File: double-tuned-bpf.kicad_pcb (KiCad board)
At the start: 2 copper layers, 52.4 x 15.6 mm, 12 parts, among them J1 PCB_SMA_EDGE, J2 PCB_SMA_EDGE, J3 Conn_01x03_Female, J4 Conn_01x03_Female, T1 6:31, T2 31:6

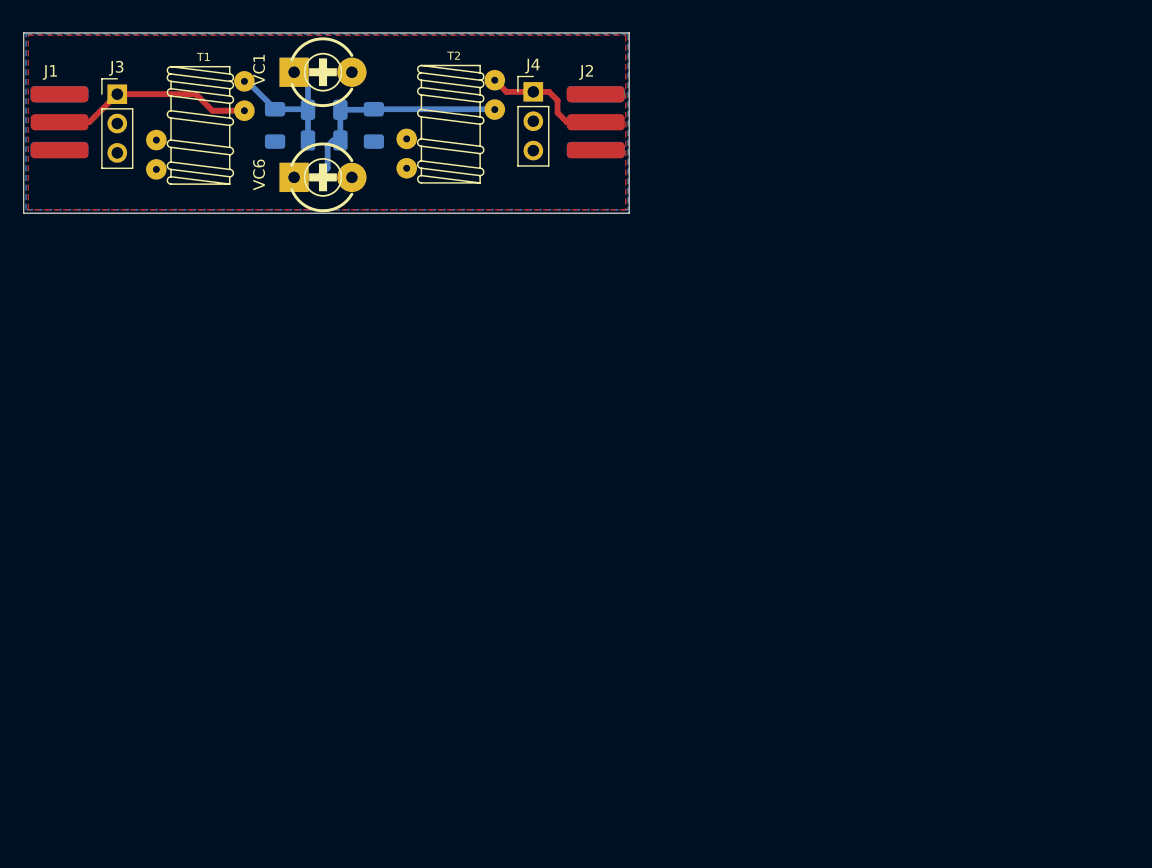
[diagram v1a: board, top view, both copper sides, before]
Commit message: gg
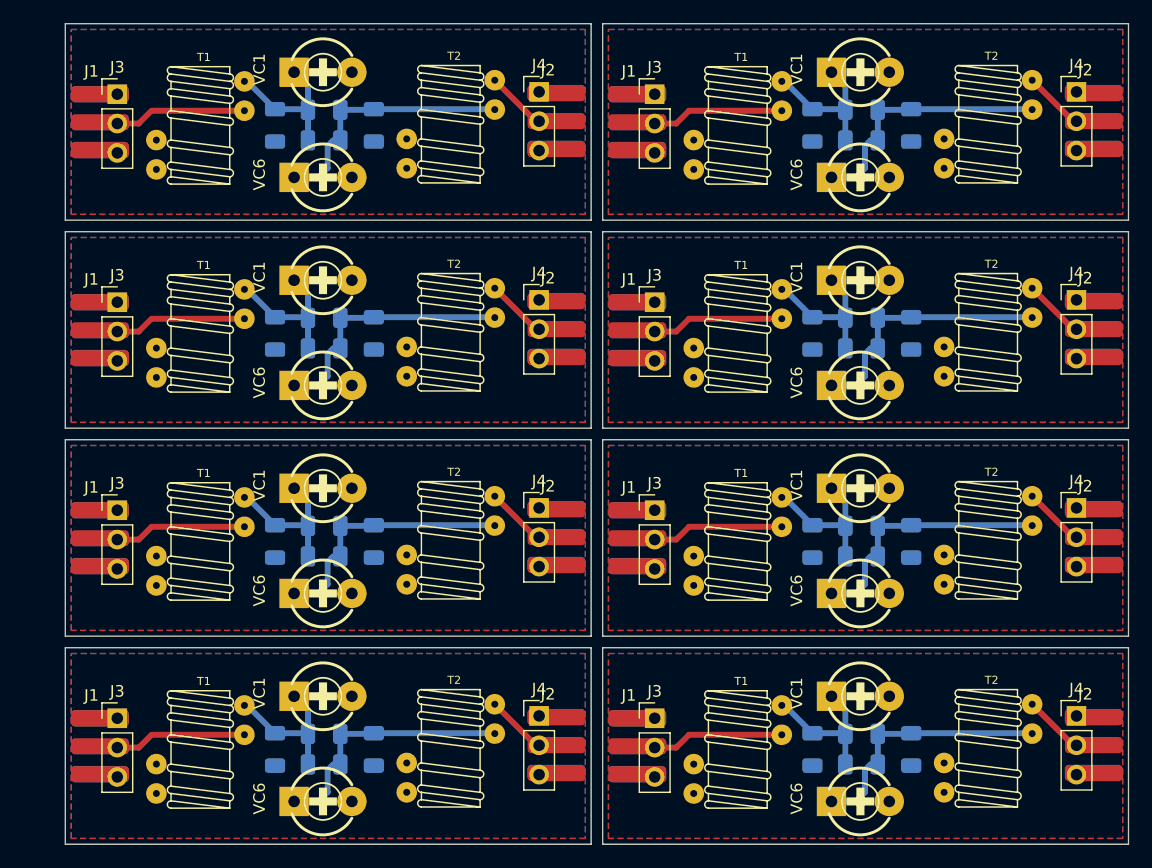
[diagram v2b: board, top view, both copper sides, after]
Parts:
- added C2: 150pF, Xenir:Capacitor 1206, B.Cu at (124.9, 133.8)
- added C2: 150pF, Xenir:Capacitor 1206, B.Cu at (171.4, 133.8)
- added C2: 150pF, Xenir:Capacitor 1206, B.Cu at (124.9, 151.8)
- added C2: 150pF, Xenir:Capacitor 1206, B.Cu at (171.4, 151.8)
- added C2: 150pF, Xenir:Capacitor 1206, B.Cu at (124.9, 115.8)
- added C2: 150pF, Xenir:Capacitor 1206, B.Cu at (171.4, 115.8)
- added C2: 150pF, Xenir:Capacitor 1206, B.Cu at (171.4, 97.8)
- added C3: 5pF, Xenir:Capacitor 1206, B.Cu at (173.4, 137.3)
- added C3: 5pF, Xenir:Capacitor 1206, B.Cu at (126.9, 137.3)
- added C3: 5pF, Xenir:Capacitor 1206, B.Cu at (173.4, 155.3)
- added C3: 5pF, Xenir:Capacitor 1206, B.Cu at (126.9, 155.3)
- added C3: 5pF, Xenir:Capacitor 1206, B.Cu at (173.4, 119.3)
- added C3: 5pF, Xenir:Capacitor 1206, B.Cu at (126.9, 119.3)
- added C3: 5pF, Xenir:Capacitor 1206, B.Cu at (173.4, 101.3)
- added C4: 10pF, Xenir:Capacitor 1206, B.Cu at (173.4, 134.7)
- added C4: 10pF, Xenir:Capacitor 1206, B.Cu at (126.9, 134.7)
- added C4: 10pF, Xenir:Capacitor 1206, B.Cu at (126.9, 152.7)
- added C4: 10pF, Xenir:Capacitor 1206, B.Cu at (173.4, 152.7)
- added C4: 10pF, Xenir:Capacitor 1206, B.Cu at (173.4, 116.7)
- added C4: 10pF, Xenir:Capacitor 1206, B.Cu at (126.9, 116.7)
- added C4: 10pF, Xenir:Capacitor 1206, B.Cu at (173.4, 98.7)
- added C5: 150pF, Xenir:Capacitor 1206, B.Cu at (133.4, 133.8)
- added C5: 150pF, Xenir:Capacitor 1206, B.Cu at (179.9, 133.8)
- added C5: 150pF, Xenir:Capacitor 1206, B.Cu at (133.4, 151.8)
- added C5: 150pF, Xenir:Capacitor 1206, B.Cu at (179.9, 151.8)
- added C5: 150pF, Xenir:Capacitor 1206, B.Cu at (133.4, 115.8)
- added C5: 150pF, Xenir:Capacitor 1206, B.Cu at (179.9, 115.8)
- added C5: 150pF, Xenir:Capacitor 1206, B.Cu at (179.9, 97.8)
- added J1: PCB_SMA_EDGE, Xenir:PCB-SMA-EDGE, F.Cu at (154.0, 146.4)
- added J1: PCB_SMA_EDGE, Xenir:PCB-SMA-EDGE, F.Cu at (107.5, 128.4)
- added J1: PCB_SMA_EDGE, Xenir:PCB-SMA-EDGE, F.Cu at (107.5, 146.4)
- added J1: PCB_SMA_EDGE, Xenir:PCB-SMA-EDGE, F.Cu at (154.0, 128.4)
- added J1: PCB_SMA_EDGE, Xenir:PCB-SMA-EDGE, F.Cu at (107.5, 110.4)
- added J1: PCB_SMA_EDGE, Xenir:PCB-SMA-EDGE, F.Cu at (154.0, 110.4)
- added J1: PCB_SMA_EDGE, Xenir:PCB-SMA-EDGE, F.Cu at (154.0, 92.4)
- added J2: PCB_SMA_EDGE, Xenir:PCB-SMA-EDGE, F.Cu at (193.5, 128.3)
- added J2: PCB_SMA_EDGE, Xenir:PCB-SMA-EDGE, F.Cu at (147.0, 128.3)
- added J2: PCB_SMA_EDGE, Xenir:PCB-SMA-EDGE, F.Cu at (193.5, 146.3)
- added J2: PCB_SMA_EDGE, Xenir:PCB-SMA-EDGE, F.Cu at (147.0, 146.3)
- added J2: PCB_SMA_EDGE, Xenir:PCB-SMA-EDGE, F.Cu at (193.5, 110.3)
- added J2: PCB_SMA_EDGE, Xenir:PCB-SMA-EDGE, F.Cu at (147.0, 110.3)
- added J2: PCB_SMA_EDGE, Xenir:PCB-SMA-EDGE, F.Cu at (193.5, 92.3)
- added J3: Conn_01x03_Female, Connector_PinHeader_2.54mm:PinHeader_1x03_P2.54mm_Vertical, F.Cu at (109.0, 131.1)
- added J3: Conn_01x03_Female, Connector_PinHeader_2.54mm:PinHeader_1x03_P2.54mm_Vertical, F.Cu at (155.5, 149.1)
- added J3: Conn_01x03_Female, Connector_PinHeader_2.54mm:PinHeader_1x03_P2.54mm_Vertical, F.Cu at (109.0, 149.1)
- added J3: Conn_01x03_Female, Connector_PinHeader_2.54mm:PinHeader_1x03_P2.54mm_Vertical, F.Cu at (155.5, 131.1)
- added J3: Conn_01x03_Female, Connector_PinHeader_2.54mm:PinHeader_1x03_P2.54mm_Vertical, F.Cu at (109.0, 113.1)
- added J3: Conn_01x03_Female, Connector_PinHeader_2.54mm:PinHeader_1x03_P2.54mm_Vertical, F.Cu at (155.5, 113.1)
- added J3: Conn_01x03_Female, Connector_PinHeader_2.54mm:PinHeader_1x03_P2.54mm_Vertical, F.Cu at (155.5, 95.1)
- added J4: Conn_01x03_Female, Connector_PinHeader_2.54mm:PinHeader_1x03_P2.54mm_Vertical, F.Cu at (192.0, 130.9)
- added J4: Conn_01x03_Female, Connector_PinHeader_2.54mm:PinHeader_1x03_P2.54mm_Vertical, F.Cu at (145.5, 130.9)
- added J4: Conn_01x03_Female, Connector_PinHeader_2.54mm:PinHeader_1x03_P2.54mm_Vertical, F.Cu at (192.0, 148.9)
- added J4: Conn_01x03_Female, Connector_PinHeader_2.54mm:PinHeader_1x03_P2.54mm_Vertical, F.Cu at (145.5, 148.9)
- added J4: Conn_01x03_Female, Connector_PinHeader_2.54mm:PinHeader_1x03_P2.54mm_Vertical, F.Cu at (192.0, 112.9)
- added J4: Conn_01x03_Female, Connector_PinHeader_2.54mm:PinHeader_1x03_P2.54mm_Vertical, F.Cu at (145.5, 112.9)
- added J4: Conn_01x03_Female, Connector_PinHeader_2.54mm:PinHeader_1x03_P2.54mm_Vertical, F.Cu at (192.0, 94.9)
- added T1: 6:31, Xenir:T37 Transformer, F.Cu at (116.2, 126.8)
- added T1: 6:31, Xenir:T37 Transformer, F.Cu at (162.7, 126.8)
- added T1: 6:31, Xenir:T37 Transformer, F.Cu at (116.2, 144.8)
- added T1: 6:31, Xenir:T37 Transformer, F.Cu at (162.7, 144.8)
- added T1: 6:31, Xenir:T37 Transformer, F.Cu at (116.2, 108.8)
- added T1: 6:31, Xenir:T37 Transformer, F.Cu at (162.7, 108.8)
- added T1: 6:31, Xenir:T37 Transformer, F.Cu at (162.7, 90.8)
- added T2: 31:6, Xenir:T37 Transformer, F.Cu at (137.9, 126.7)
- added T2: 31:6, Xenir:T37 Transformer, F.Cu at (137.9, 144.7)
- added T2: 31:6, Xenir:T37 Transformer, F.Cu at (184.4, 144.7)
- added T2: 31:6, Xenir:T37 Transformer, F.Cu at (184.4, 126.7)
- added T2: 31:6, Xenir:T37 Transformer, F.Cu at (137.9, 108.7)
- added T2: 31:6, Xenir:T37 Transformer, F.Cu at (184.4, 108.7)
- added T2: 31:6, Xenir:T37 Transformer, F.Cu at (184.4, 90.7)
- added VC1: 40pF, Xenir:trimcap, F.Cu at (120.3, 129.2)
- added VC1: 40pF, Xenir:trimcap, F.Cu at (166.8, 147.2)
- added VC1: 40pF, Xenir:trimcap, F.Cu at (120.3, 147.2)
- added VC1: 40pF, Xenir:trimcap, F.Cu at (166.8, 129.2)
- added VC1: 40pF, Xenir:trimcap, F.Cu at (120.3, 111.2)
- added VC1: 40pF, Xenir:trimcap, F.Cu at (166.8, 111.2)
- added VC1: 40pF, Xenir:trimcap, F.Cu at (166.8, 93.2)
- added VC6: 40pF, Xenir:trimcap, F.Cu at (120.3, 138.3)
- added VC6: 40pF, Xenir:trimcap, F.Cu at (166.8, 138.3)
- added VC6: 40pF, Xenir:trimcap, F.Cu at (166.8, 156.3)
- added VC6: 40pF, Xenir:trimcap, F.Cu at (120.3, 156.3)
- added VC6: 40pF, Xenir:trimcap, F.Cu at (120.3, 120.3)
- added VC6: 40pF, Xenir:trimcap, F.Cu at (166.8, 120.3)
- added VC6: 40pF, Xenir:trimcap, F.Cu at (166.8, 102.3)
- moved J1 3.50 mm to (107.5, 92.4)
- moved J2 3.40 mm to (147.0, 92.3)
- moved J4 0.50 mm to (145.5, 94.9)
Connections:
- J3 pad 1: Input -> GND
- J3 pad 2: (no net) -> Input
- J4 pad 1: Output -> GND
- J4 pad 2: (no net) -> Output
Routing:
- net (no net): track 0.00 -> 366.6 mm
- net Input: track 17.6 -> 11.5 mm
- net Output: track 10.9 -> 5.31 mm
- added copper zone on B.Cu, net (none)
- added copper zone on F.Cu, net (none)
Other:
- board size 52.4 x 15.6 mm -> 92 x 71 mm
